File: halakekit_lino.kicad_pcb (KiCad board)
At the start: 2 copper layers, 33 x 20.6 mm, 10 parts, among them J1 HEADER_3, J2 HEADER_3, J3 HEADER_3, J4 HEADER_3, U1 BCM20737S

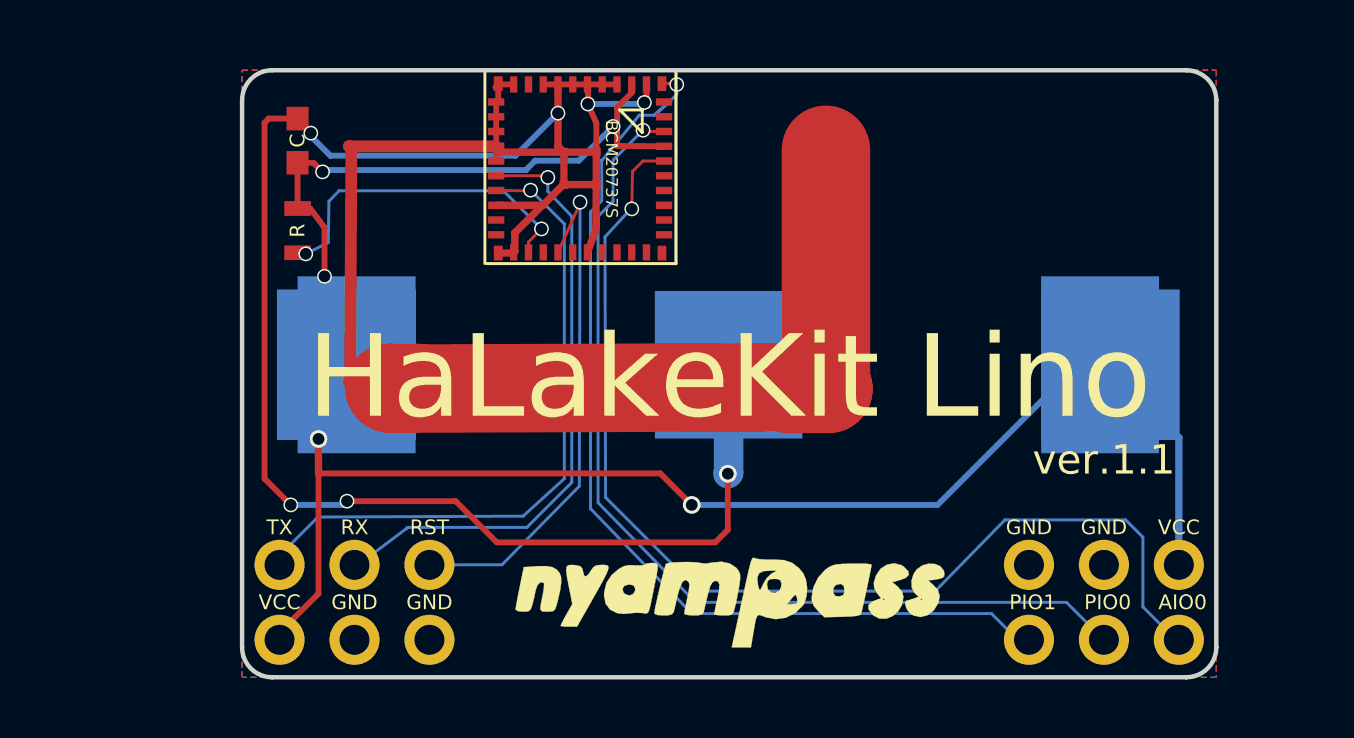
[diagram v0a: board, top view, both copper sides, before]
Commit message: Change board layout as rev 1.2
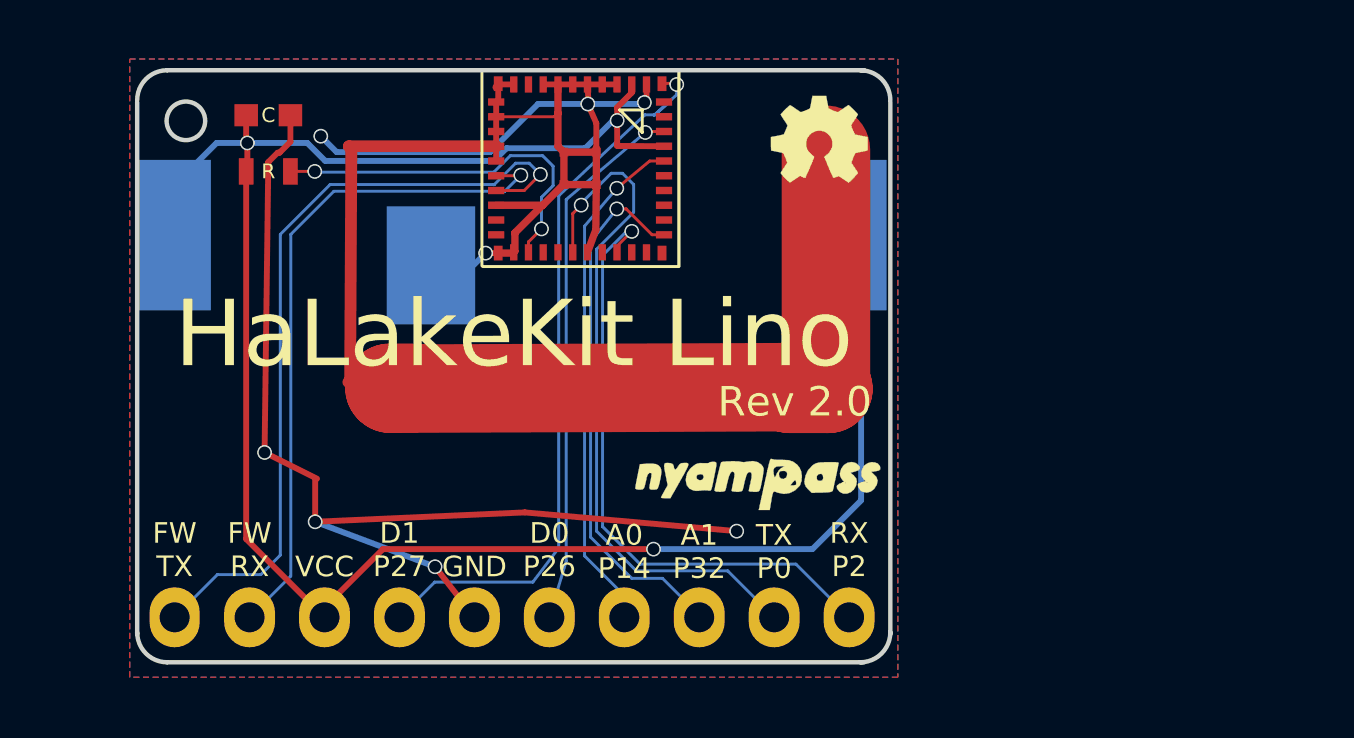
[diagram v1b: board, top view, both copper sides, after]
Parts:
- removed the G*** at (164.1, 110.9)
- removed J2, J3, J4: HEADER_3, simple_headers:Pin_Header_Straight_1x03_circle
- added G***: LOGO, osh-logo:osh-logo-4p3mm, F.Cu at (177.3, 100.8)
- added G***: LOGO, osh-logo:osh-logo-4p3mm, F.Cu at (174.5, 99.2)
- added G***: LOGO, osh-logo:osh-logo-3p4mm, F.Cu at (167.2, 95.2)
- added G***: LOGO, osh-logo:osh-logo-3p4mm, B.Cu at (167.4, 104.1)
- added G***: LOGO, logos:nyampass_logo_8p4mm, F.Cu at (165.1, 106.9)
- BT1: footprint CR2032_frame:BC-2001(CR2032 frame) -> CR2032_frame:BAT-HLD-001-TRCT
- J1: value HEADER_3 -> HEADER_10; footprint simple_headers:Pin_Header_Straight_1x03_circle -> simple_headers:Pin_Header_Straight_1x10
- moved G*** 17.9 mm to (165.1, 107.0), turned to 0 degrees
- moved J1 8.82 mm to (145.3, 111.4), turned to 90 degrees
- moved BT1 7.13 mm to (156.7, 98.5)
- moved R 2.24 mm to (148.5, 96.3), turned to 0 degrees
- moved C 1.31 mm to (148.5, 94.4), turned to 0 degrees
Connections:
- J1 pad 1: RST -> FWTX
- J1 pad 2: RX -> FWRX
- J1 pad 3: TX -> VCC
- U1 pad 1: PIO1 -> D1
- U1 pad 18: RX -> FWRX
- U1 pad 19: TX -> FWTX
- U1 pad 27: RST -> Net-(U1-Pad27)
- U1 pad 28: Net-(U1-Pad28) -> TX
- U1 pad 31: Net-(U1-Pad31) -> RX
- U1 pad 35: Net-(U1-Pad35) -> A1
- U1 pad 40: AIO -> A0
- U1 pad 42: PIO0 -> D0
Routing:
- net AIO: track 37.6 -> 0.00 mm, vias 1 -> 0
- net PIO1: track 33.7 -> 0.00 mm, vias 1 -> 0
- net PIO0: track 33.1 -> 0.00 mm, vias 1 -> 0
- net FWTX: track 0.00 -> 27.0 mm, vias 0 -> 1
- net D1: track 0.00 -> 25.2 mm, vias 0 -> 1
- net FWRX: track 0.00 -> 23.1 mm, vias 0 -> 1
- net D0: track 0.00 -> 18.4 mm, vias 0 -> 1
- net A1: track 0.00 -> 18.3 mm, vias 0 -> 1
- net RST: track 17.7 -> 0.00 mm, vias 1 -> 0
- net A0: track 0.00 -> 17.4 mm, vias 0 -> 1
- net VCC: track 73.2 -> 69.4 mm, vias 5 -> 3
- net TX: track 22.4 -> 23.6 mm
- net Net-(10K1-Pad2): track 11.4 -> 12.6 mm
- net GND: track 115.3 -> 115.4 mm, vias 7 -> 8
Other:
- board size 33 x 20.6 mm -> 25.5 x 20.1 mm
- net class GND added: clearance 0.1, trace_width 0.2, via_dia 0.5, via_drill 0.4
- net class VCC added: clearance 0.1, trace_width 0.2, via_dia 0.5, via_drill 0.4
- board text added: "A0 P14"
- board text added: "A1 P32"
- board text added: "D0 P26"
- board text added: "D1 D27"
- board text added: "D1 P27"
- board text added: "FW RX"
- board text added: "FW TX"
- board text added: "HaLakeKit"
- board text added: "Lino"
- board text added: "RX P2"
- board text added: "Rev 2.0"
- board text added: "TX P0"
- board text removed: "AIO0"
- board text removed: "BCM20737S"
- board text removed: "PIO0"
- board text removed: "PIO1"
- board text removed: "RST"
- board text removed: "RX"
- board text removed: "TX"
- board text removed: "ver.1.1"
